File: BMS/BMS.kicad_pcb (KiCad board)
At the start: 2 copper layers, 57.4 x 167.7 mm, 5 parts

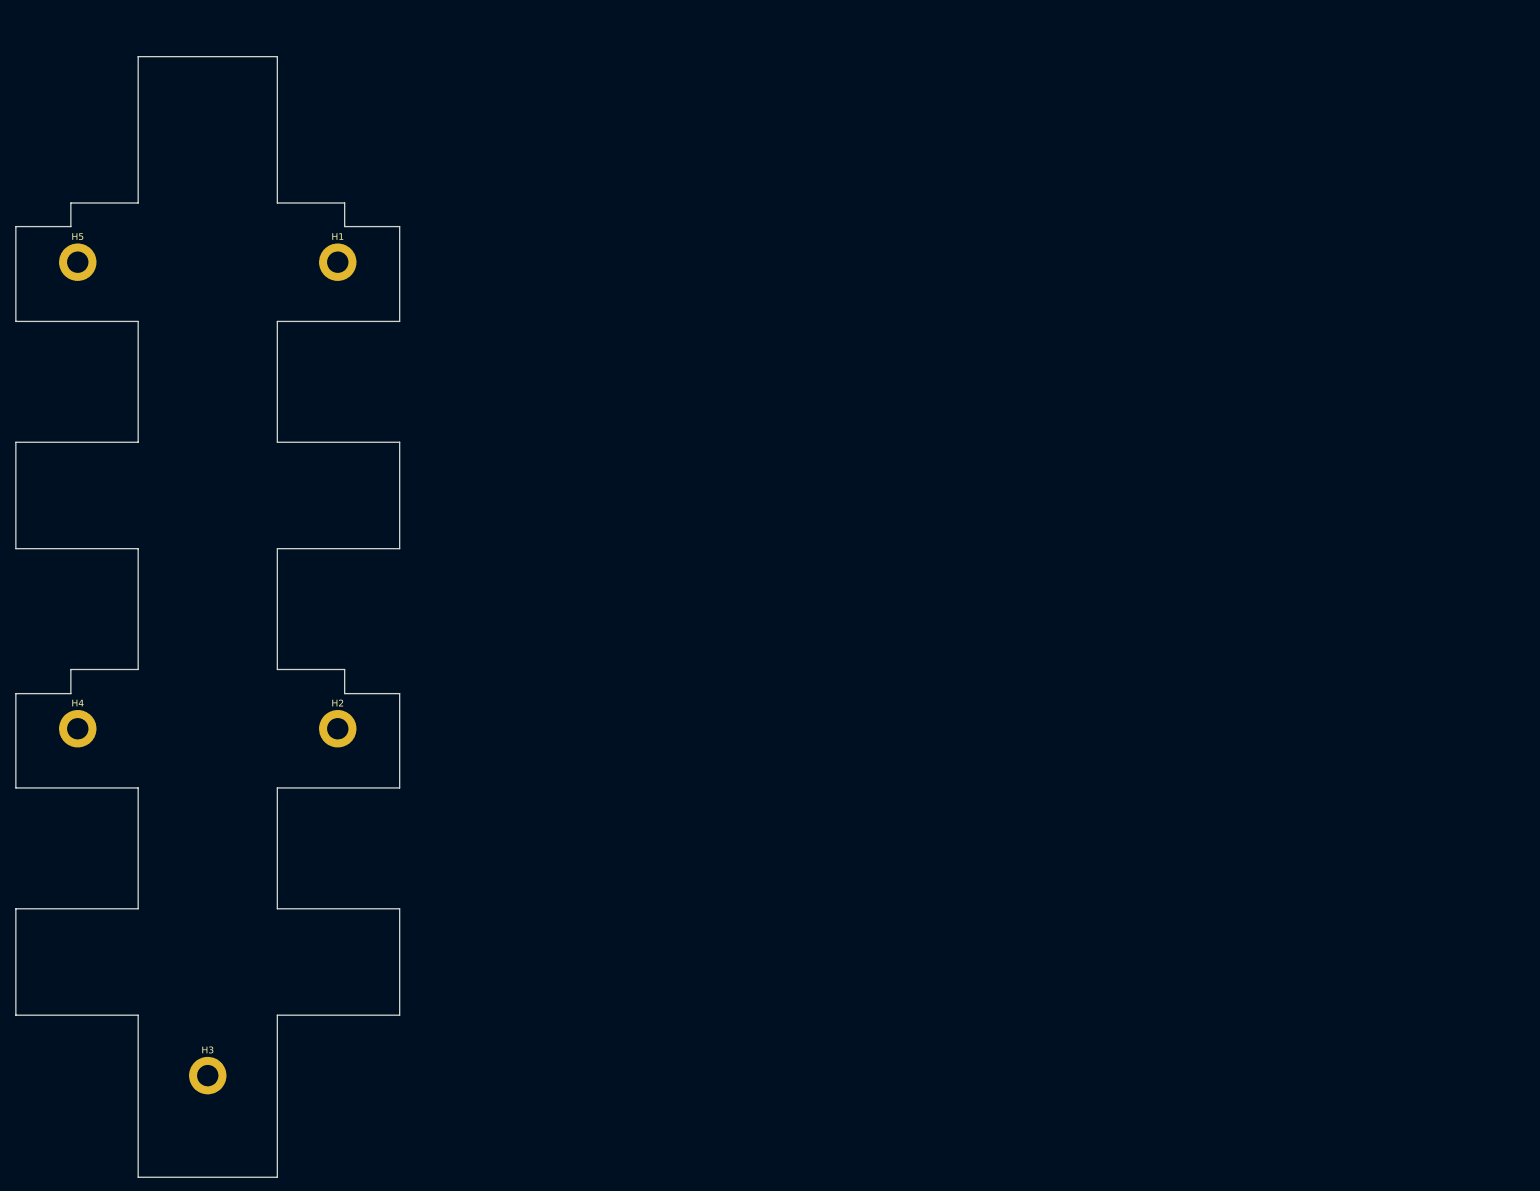
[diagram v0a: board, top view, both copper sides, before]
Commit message: bms pcb blocked (for rn)
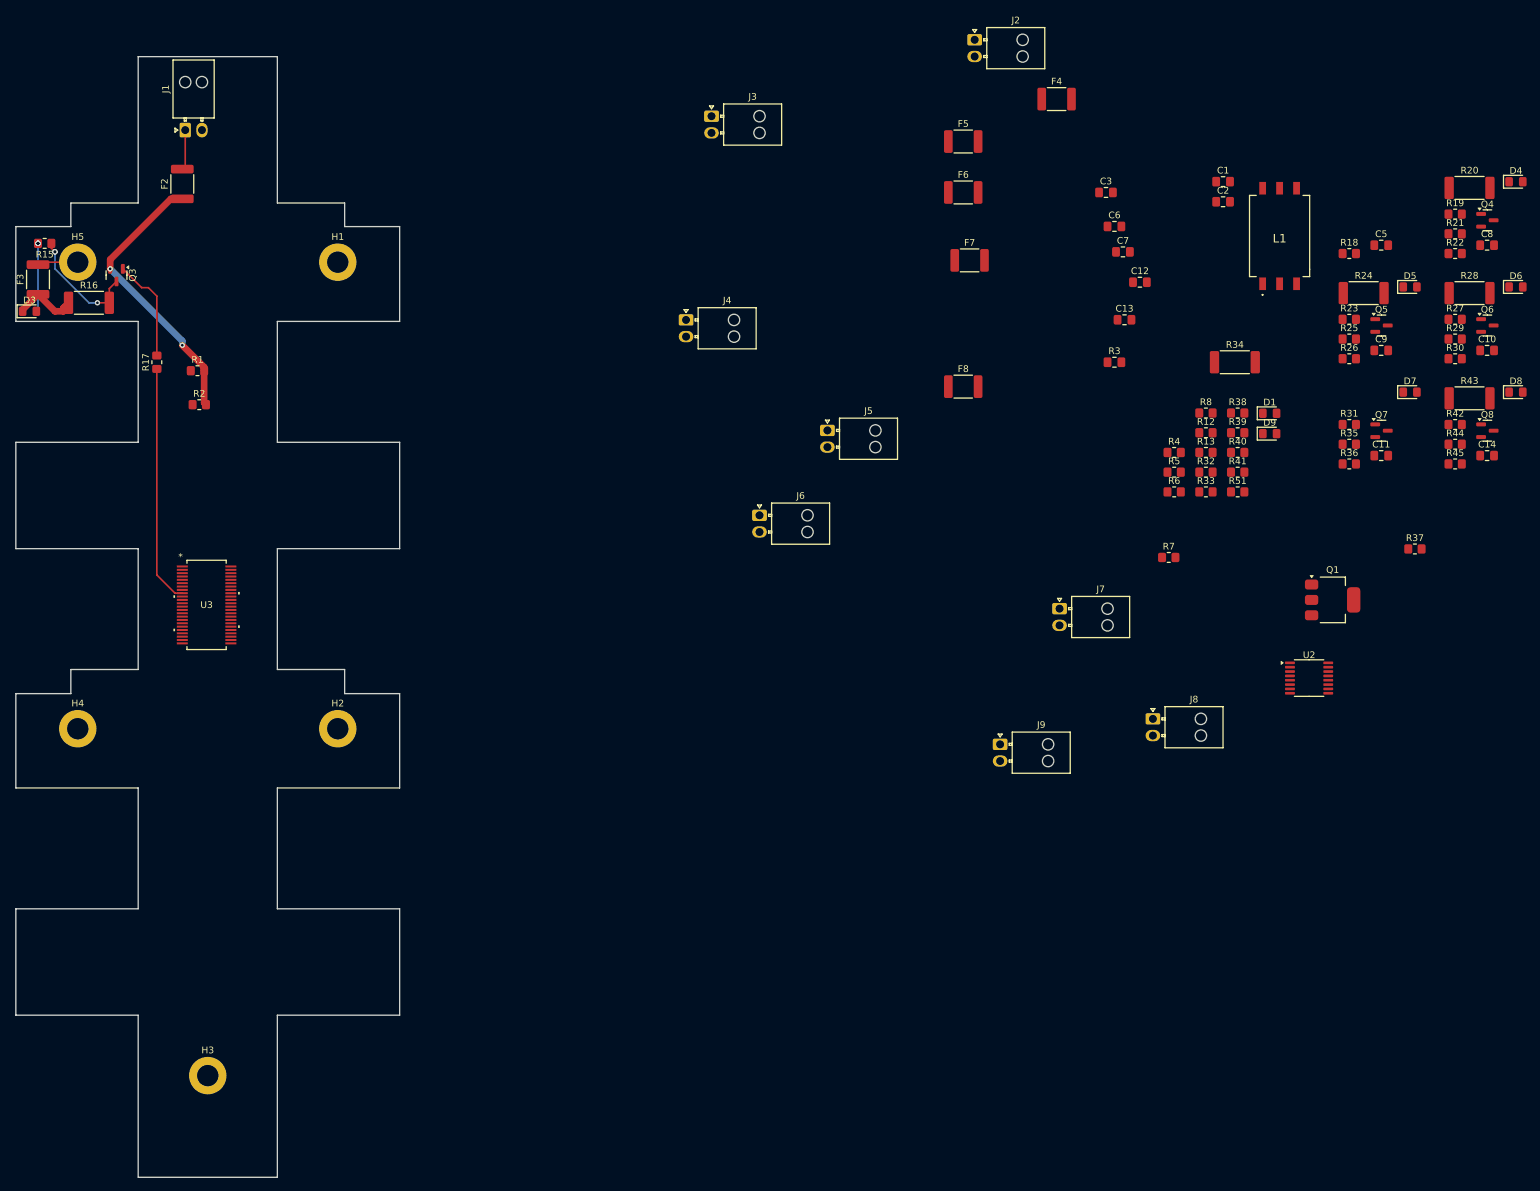
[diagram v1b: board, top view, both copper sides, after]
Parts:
- added C1: 100nF, Capacitor_SMD:C_0805_2012Metric_Pad1.18x1.45mm_HandSolder, F.Cu at (202.7, 44.1)
- added C10: 10nF, Capacitor_SMD:C_0805_2012Metric_Pad1.18x1.45mm_HandSolder, F.Cu at (242.2, 69.3)
- added C11: 10nF, Capacitor_SMD:C_0805_2012Metric_Pad1.18x1.45mm_HandSolder, F.Cu at (226.4, 85.1)
- added C12: 15pF, Capacitor_SMD:C_0805_2012Metric_Pad1.18x1.45mm_HandSolder, F.Cu at (190.3, 59.1)
- added C13: 10nF, Capacitor_SMD:C_0805_2012Metric_Pad1.18x1.45mm_HandSolder, F.Cu at (188.0, 64.8)
- added C14: 10nF, Capacitor_SMD:C_0805_2012Metric_Pad1.18x1.45mm_HandSolder, F.Cu at (242.2, 85.1)
- added C2: 10nF, Capacitor_SMD:C_0805_2012Metric_Pad1.18x1.45mm_HandSolder, F.Cu at (202.7, 47.1)
- added C3: 1uF, Capacitor_SMD:C_0805_2012Metric_Pad1.18x1.45mm_HandSolder, F.Cu at (185.2, 45.7)
- added C5: 10nF, Capacitor_SMD:C_0805_2012Metric_Pad1.18x1.45mm_HandSolder, F.Cu at (226.4, 53.6)
- added C6: 1uF, Capacitor_SMD:C_0805_2012Metric_Pad1.18x1.45mm_HandSolder, F.Cu at (186.5, 50.8)
- added C7: 1uF, Capacitor_SMD:C_0805_2012Metric_Pad1.18x1.45mm_HandSolder, F.Cu at (187.7, 54.6)
- added C8: 10nF, Capacitor_SMD:C_0805_2012Metric_Pad1.18x1.45mm_HandSolder, F.Cu at (242.2, 53.6)
- added C9: 10nF, Capacitor_SMD:C_0805_2012Metric_Pad1.18x1.45mm_HandSolder, F.Cu at (226.4, 69.3)
- added D1: LH R974-LP-1, LED_SMD:LED_0805_2012Metric_Pad1.15x1.40mm_HandSolder, F.Cu at (209.7, 78.8)
- added D3: LH R974-LP-1, LED_SMD:LED_0805_2012Metric_Pad1.15x1.40mm_HandSolder, F.Cu at (24.1, 63.5)
- added D4: LH R974-LP-1, LED_SMD:LED_0805_2012Metric_Pad1.15x1.40mm_HandSolder, F.Cu at (246.5, 44.1)
- added D5: LH R974-LP-1, LED_SMD:LED_0805_2012Metric_Pad1.15x1.40mm_HandSolder, F.Cu at (230.7, 59.9)
- added D6: LH R974-LP-1, LED_SMD:LED_0805_2012Metric_Pad1.15x1.40mm_HandSolder, F.Cu at (246.5, 59.9)
- added D7: LH R974-LP-1, LED_SMD:LED_0805_2012Metric_Pad1.15x1.40mm_HandSolder, F.Cu at (230.7, 75.6)
- added D8: LH R974-LP-1, LED_SMD:LED_0805_2012Metric_Pad1.15x1.40mm_HandSolder, F.Cu at (246.5, 75.6)
- added D9: LH R974-LP-1, LED_SMD:LED_0805_2012Metric_Pad1.15x1.40mm_HandSolder, F.Cu at (209.7, 81.8)
- added F2: Polyfuse, Fuse:Fuse_1812_4532Metric_Pad1.30x3.40mm_HandSolder, F.Cu at (47.0, 44.5)
- added F3: Polyfuse, Fuse:Fuse_1812_4532Metric_Pad1.30x3.40mm_HandSolder, F.Cu at (25.4, 58.7)
- added F4: Polyfuse, Fuse:Fuse_1812_4532Metric_Pad1.30x3.40mm_HandSolder, F.Cu at (177.8, 31.8)
- added F5: Polyfuse, Fuse:Fuse_1812_4532Metric_Pad1.30x3.40mm_HandSolder, F.Cu at (163.8, 38.1)
- added F6: Polyfuse, Fuse:Fuse_1812_4532Metric_Pad1.30x3.40mm_HandSolder, F.Cu at (163.8, 45.7)
- added F7: Polyfuse, Fuse:Fuse_1812_4532Metric_Pad1.30x3.40mm_HandSolder, F.Cu at (164.8, 55.9)
- added F8: Polyfuse, Fuse:Fuse_1812_4532Metric_Pad1.30x3.40mm_HandSolder, F.Cu at (163.8, 74.8)
- added J1: Conn_01x02_Pin, Connector_Molex:Molex_Nano-Fit_105313-xx02_1x02_P2.50mm_Horizontal, F.Cu at (47.4, 36.4)
- added J2: IsoSPI, Connector_Molex:Molex_Nano-Fit_105313-xx02_1x02_P2.50mm_Horizontal, F.Cu at (165.5, 22.9)
- added J3: IsoSPI, Connector_Molex:Molex_Nano-Fit_105313-xx02_1x02_P2.50mm_Horizontal, F.Cu at (126.2, 34.3)
- added J4: ~, Connector_Molex:Molex_Nano-Fit_105313-xx02_1x02_P2.50mm_Horizontal, F.Cu at (122.4, 64.8)
- added J5: ~, Connector_Molex:Molex_Nano-Fit_105313-xx02_1x02_P2.50mm_Horizontal, F.Cu at (143.5, 81.3)
- added J6: ~, Connector_Molex:Molex_Nano-Fit_105313-xx02_1x02_P2.50mm_Horizontal, F.Cu at (133.3, 94.0)
- added J7: ~, Connector_Molex:Molex_Nano-Fit_105313-xx02_1x02_P2.50mm_Horizontal, F.Cu at (178.2, 108.0)
- added J8: ~, Connector_Molex:Molex_Nano-Fit_105313-xx02_1x02_P2.50mm_Horizontal, F.Cu at (192.2, 124.5)
- added J9: ~, Connector_Molex:Molex_Nano-Fit_105313-xx02_1x02_P2.50mm_Horizontal, F.Cu at (169.3, 128.3)
- added L1: HM2113ZNL, FS_3_Global_Footprint_Library:HM2113ZNLT, F.Cu at (211.2, 52.2)
- added Q1: NSV1C201MZ4, Package_TO_SOT_SMD:SOT-223, F.Cu at (219.1, 106.7)
- added Q3: BSS308PE, Package_TO_SOT_SMD:SOT-23, F.Cu at (37.1, 58.1)
- added Q4: BSS308PE, Package_TO_SOT_SMD:SOT-23, F.Cu at (242.2, 49.9)
- added Q5: BSS308PE, Package_TO_SOT_SMD:SOT-23, F.Cu at (226.4, 65.6)
- added Q6: BSS308PE, Package_TO_SOT_SMD:SOT-23, F.Cu at (242.2, 65.6)
- added Q7: BSS308PE, Package_TO_SOT_SMD:SOT-23, F.Cu at (226.4, 81.4)
- added Q8: BSS308PE, Package_TO_SOT_SMD:SOT-23, F.Cu at (242.2, 81.4)
- added R1: 100, Resistor_SMD:R_0805_2012Metric_Pad1.20x1.40mm_HandSolder, F.Cu at (49.3, 72.4)
- added R12: 1.5k, Resistor_SMD:R_0805_2012Metric_Pad1.20x1.40mm_HandSolder, F.Cu at (200.1, 81.7)
- added R13: 680, Resistor_SMD:R_0805_2012Metric_Pad1.20x1.40mm_HandSolder, F.Cu at (200.1, 84.6)
- added R15: 120, Resistor_SMD:R_0805_2012Metric_Pad1.20x1.40mm_HandSolder, F.Cu at (26.4, 53.3)
- added R16: 33, Resistor_SMD:R_2512_6332Metric_Pad1.40x3.35mm_HandSolder, F.Cu at (33.0, 62.2)
- added R17: 3.3k, Resistor_SMD:R_0805_2012Metric_Pad1.20x1.40mm_HandSolder, F.Cu at (43.2, 71.1)
- added R18: 100, Resistor_SMD:R_0805_2012Metric_Pad1.20x1.40mm_HandSolder, F.Cu at (221.6, 54.9)
- added R19: 120, Resistor_SMD:R_0805_2012Metric_Pad1.20x1.40mm_HandSolder, F.Cu at (237.4, 49.0)
- added R2: 100, Resistor_SMD:R_0805_2012Metric_Pad1.20x1.40mm_HandSolder, F.Cu at (49.5, 77.5)
- added R20: 33, Resistor_SMD:R_2512_6332Metric_Pad1.40x3.35mm_HandSolder, F.Cu at (239.6, 45.0)
- added R21: 3.3k, Resistor_SMD:R_0805_2012Metric_Pad1.20x1.40mm_HandSolder, F.Cu at (237.4, 51.9)
- added R22: 100, Resistor_SMD:R_0805_2012Metric_Pad1.20x1.40mm_HandSolder, F.Cu at (237.4, 54.9)
- added R23: 120, Resistor_SMD:R_0805_2012Metric_Pad1.20x1.40mm_HandSolder, F.Cu at (221.6, 64.7)
- added R24: 33, Resistor_SMD:R_2512_6332Metric_Pad1.40x3.35mm_HandSolder, F.Cu at (223.7, 60.8)
- added R25: 3.3k, Resistor_SMD:R_0805_2012Metric_Pad1.20x1.40mm_HandSolder, F.Cu at (221.6, 67.7)
- added R26: 100, Resistor_SMD:R_0805_2012Metric_Pad1.20x1.40mm_HandSolder, F.Cu at (221.6, 70.6)
- added R27: 120, Resistor_SMD:R_0805_2012Metric_Pad1.20x1.40mm_HandSolder, F.Cu at (237.4, 64.7)
- added R28: 33, Resistor_SMD:R_2512_6332Metric_Pad1.40x3.35mm_HandSolder, F.Cu at (239.6, 60.8)
- added R29: 3.3k, Resistor_SMD:R_0805_2012Metric_Pad1.20x1.40mm_HandSolder, F.Cu at (237.4, 67.7)
- added R3: 100, Capacitor_SMD:C_0805_2012Metric_Pad1.18x1.45mm_HandSolder, F.Cu at (186.5, 71.1)
- added R30: 100, Resistor_SMD:R_0805_2012Metric_Pad1.20x1.40mm_HandSolder, F.Cu at (237.4, 70.6)
- added R31: 120, Resistor_SMD:R_0805_2012Metric_Pad1.20x1.40mm_HandSolder, F.Cu at (221.6, 80.4)
- added R32: 402, Resistor_SMD:R_0805_2012Metric_Pad1.20x1.40mm_HandSolder, F.Cu at (200.1, 87.6)
- added R33: 2.2k, Resistor_SMD:R_0805_2012Metric_Pad1.20x1.40mm_HandSolder, F.Cu at (200.1, 90.5)
- added R34: 33, Resistor_SMD:R_2512_6332Metric_Pad1.40x3.35mm_HandSolder, F.Cu at (204.5, 71.1)
- added R35: 3.3k, Resistor_SMD:R_0805_2012Metric_Pad1.20x1.40mm_HandSolder, F.Cu at (221.6, 83.4)
- added R36: 100, Resistor_SMD:R_0805_2012Metric_Pad1.20x1.40mm_HandSolder, F.Cu at (221.6, 86.3)
- added R37: 10k, Resistor_SMD:R_0805_2012Metric_Pad1.20x1.40mm_HandSolder, F.Cu at (231.4, 99.1)
- added R38: 10k, Resistor_SMD:R_0805_2012Metric_Pad1.20x1.40mm_HandSolder, F.Cu at (204.9, 78.7)
- added R39: 10k, Resistor_SMD:R_0805_2012Metric_Pad1.20x1.40mm_HandSolder, F.Cu at (204.9, 81.7)
- added R4: 10k, Resistor_SMD:R_0805_2012Metric_Pad1.20x1.40mm_HandSolder, F.Cu at (195.4, 84.6)
- added R40: 22, Resistor_SMD:R_0805_2012Metric_Pad1.20x1.40mm_HandSolder, F.Cu at (204.9, 84.6)
- added R41: 22, Resistor_SMD:R_0805_2012Metric_Pad1.20x1.40mm_HandSolder, F.Cu at (204.9, 87.6)
- added R42: 120, Resistor_SMD:R_0805_2012Metric_Pad1.20x1.40mm_HandSolder, F.Cu at (237.4, 80.4)
- added R43: 33, Resistor_SMD:R_2512_6332Metric_Pad1.40x3.35mm_HandSolder, F.Cu at (239.6, 76.5)
- added R44: 3.3k, Resistor_SMD:R_0805_2012Metric_Pad1.20x1.40mm_HandSolder, F.Cu at (237.4, 83.4)
- added R45: 100, Resistor_SMD:R_0805_2012Metric_Pad1.20x1.40mm_HandSolder, F.Cu at (237.4, 86.3)
- added R5: 200, Resistor_SMD:R_0805_2012Metric_Pad1.20x1.40mm_HandSolder, F.Cu at (195.4, 87.6)
- added R51: 160, Resistor_SMD:R_0805_2012Metric_Pad1.20x1.40mm_HandSolder, F.Cu at (204.9, 90.5)
- added R6: 160, Resistor_SMD:R_0805_2012Metric_Pad1.20x1.40mm_HandSolder, F.Cu at (195.4, 90.5)
- added R7: 10k, Resistor_SMD:R_0805_2012Metric_Pad1.20x1.40mm_HandSolder, F.Cu at (194.6, 100.3)
- added R8: 10k, Resistor_SMD:R_0805_2012Metric_Pad1.20x1.40mm_HandSolder, F.Cu at (200.1, 78.7)
- added U2: ADG708, Package_SO:TSSOP-16_4.4x5mm_P0.65mm, F.Cu at (215.6, 118.4)
- added U3: LTC6811IG-2-TRPBF, FS_3_Global_Footprint_Library:LTC6811-2, F.Cu at (50.6, 107.4)
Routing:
- net /BB5/B#+1: track 0.00 -> 42.2 mm, vias 0 -> 2
- net /S9: track 0.00 -> 35.8 mm
- net Net-(Q3-D): track 0.00 -> 17.9 mm, vias 0 -> 3
- net Net-(Q3-G): track 0.00 -> 15.7 mm
- net Net-(D3-A): track 0.00 -> 10.2 mm, vias 0 -> 4
- net /BB4/B#+1: track 0.00 -> 9.94 mm
- net Net-(F3-Pad2): track 0.00 -> 6.10 mm
- net Net-(J1-Pin_1): track 0.00 -> 6.02 mm

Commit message: Fixed footprints and 3d models for bms
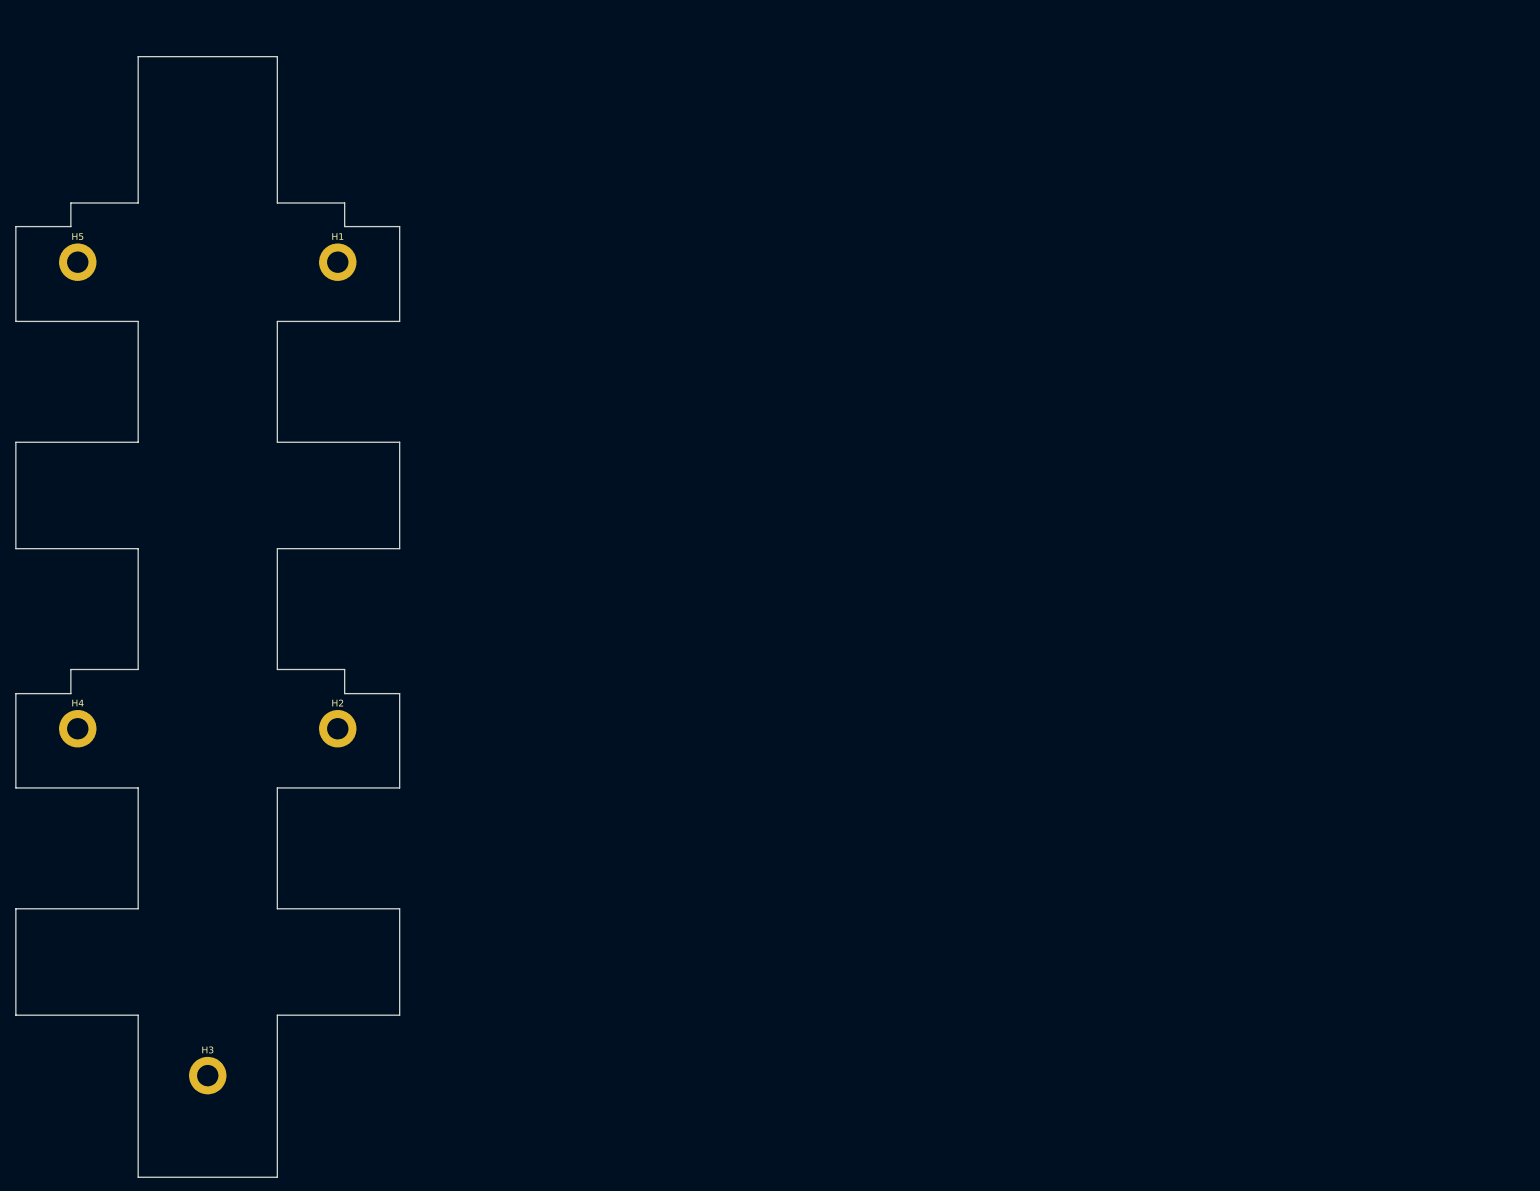
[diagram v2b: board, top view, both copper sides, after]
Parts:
- removed C1: 100nF, Capacitor_SMD:C_0805_2012Metric_Pad1.18x1.45mm_HandSolder
- removed C10, C11, C13, C14, C2, C5, C8, C9: 10nF, Capacitor_SMD:C_0805_2012Metric_Pad1.18x1.45mm_HandSolder
- removed C12: 15pF, Capacitor_SMD:C_0805_2012Metric_Pad1.18x1.45mm_HandSolder
- removed C3, C6, C7: 1uF, Capacitor_SMD:C_0805_2012Metric_Pad1.18x1.45mm_HandSolder
- removed D1, D3, D4, D5, D6, D7, D8, D9: LH R974-LP-1, LED_SMD:LED_0805_2012Metric_Pad1.15x1.40mm_HandSolder
- removed F2, F3, F4, F5, F6, F7, F8: Polyfuse, Fuse:Fuse_1812_4532Metric_Pad1.30x3.40mm_HandSolder
- removed J1: Conn_01x02_Pin, Connector_Molex:Molex_Nano-Fit_105313-xx02_1x02_P2.50mm_Horizontal
- removed J2, J3: IsoSPI, Connector_Molex:Molex_Nano-Fit_105313-xx02_1x02_P2.50mm_Horizontal
- removed J4, J5, J6, J7, J8, J9: ~, Connector_Molex:Molex_Nano-Fit_105313-xx02_1x02_P2.50mm_Horizontal
- removed L1: HM2113ZNL, FS_3_Global_Footprint_Library:HM2113ZNLT
- removed Q1: NSV1C201MZ4, Package_TO_SOT_SMD:SOT-223
- removed Q3, Q4, Q5, Q6, Q7, Q8: BSS308PE, Package_TO_SOT_SMD:SOT-23
- removed R1, R18, R2, R22, R26, R30, R36, R45: 100, Resistor_SMD:R_0805_2012Metric_Pad1.20x1.40mm_HandSolder
- removed R12: 1.5k, Resistor_SMD:R_0805_2012Metric_Pad1.20x1.40mm_HandSolder
- removed R13: 680, Resistor_SMD:R_0805_2012Metric_Pad1.20x1.40mm_HandSolder
- removed R15, R19, R23, R27, R31, R42: 120, Resistor_SMD:R_0805_2012Metric_Pad1.20x1.40mm_HandSolder
- removed R16, R20, R24, R28, R34, R43: 33, Resistor_SMD:R_2512_6332Metric_Pad1.40x3.35mm_HandSolder
- removed R17, R21, R25, R29, R35, R44: 3.3k, Resistor_SMD:R_0805_2012Metric_Pad1.20x1.40mm_HandSolder
- removed R3: 100, Capacitor_SMD:C_0805_2012Metric_Pad1.18x1.45mm_HandSolder
- removed R32: 402, Resistor_SMD:R_0805_2012Metric_Pad1.20x1.40mm_HandSolder
- removed R33: 2.2k, Resistor_SMD:R_0805_2012Metric_Pad1.20x1.40mm_HandSolder
- removed R37, R38, R39, R4, R7, R8: 10k, Resistor_SMD:R_0805_2012Metric_Pad1.20x1.40mm_HandSolder
- removed R40, R41: 22, Resistor_SMD:R_0805_2012Metric_Pad1.20x1.40mm_HandSolder
- removed R5: 200, Resistor_SMD:R_0805_2012Metric_Pad1.20x1.40mm_HandSolder
- removed R51, R6: 160, Resistor_SMD:R_0805_2012Metric_Pad1.20x1.40mm_HandSolder
- removed U2: ADG708, Package_SO:TSSOP-16_4.4x5mm_P0.65mm
- removed U3: LTC6811IG-2-TRPBF, FS_3_Global_Footprint_Library:LTC6811-2
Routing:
- net /BB5/B#+1: track 42.2 -> 0.00 mm, vias 2 -> 0
- net /S9: track 35.8 -> 0.00 mm
- net Net-(Q3-D): track 17.9 -> 0.00 mm, vias 3 -> 0
- net Net-(Q3-G): track 15.7 -> 0.00 mm
- net Net-(D3-A): track 10.2 -> 0.00 mm, vias 4 -> 0
- net /BB4/B#+1: track 9.94 -> 0.00 mm
- net Net-(F3-Pad2): track 6.10 -> 0.00 mm
- net Net-(J1-Pin_1): track 6.02 -> 0.00 mm
